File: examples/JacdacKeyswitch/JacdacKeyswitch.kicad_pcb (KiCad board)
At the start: 2 copper layers, 35 x 25 mm, 37 parts

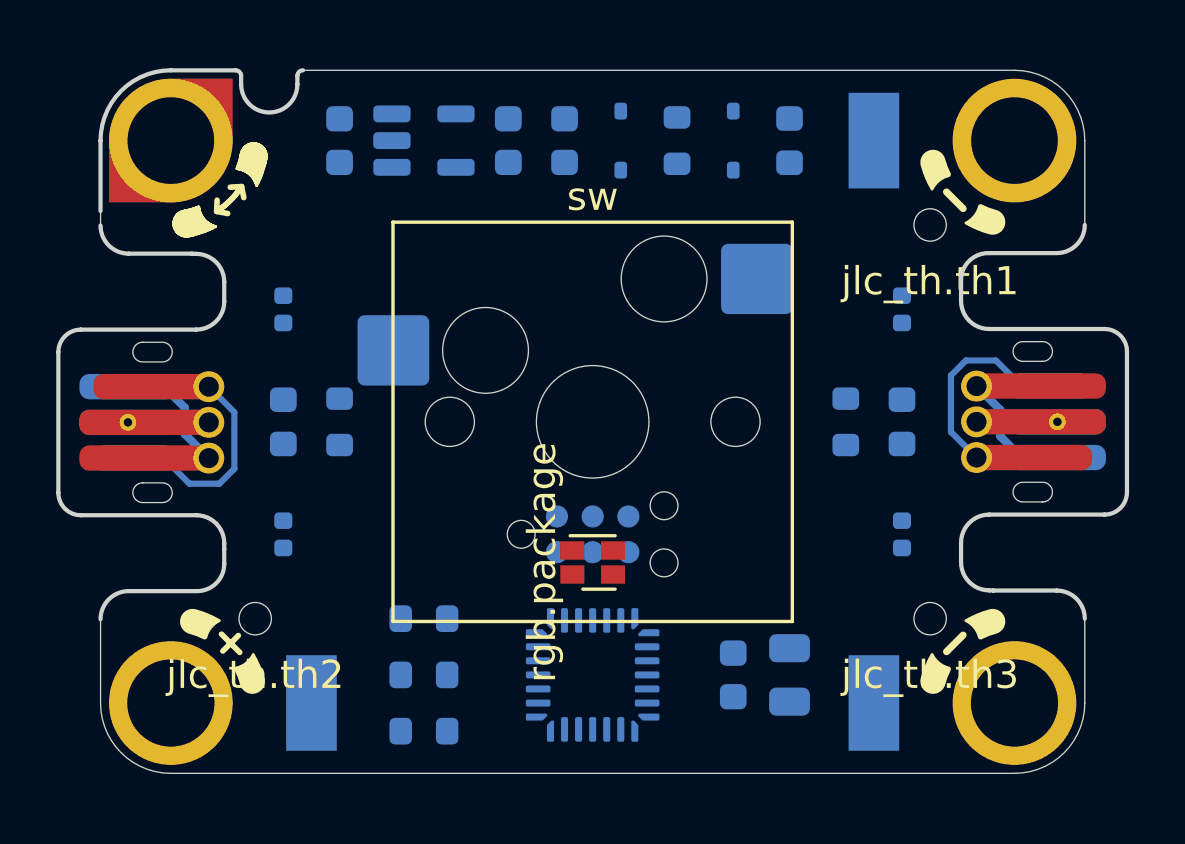
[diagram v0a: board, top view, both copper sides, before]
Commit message: layout!
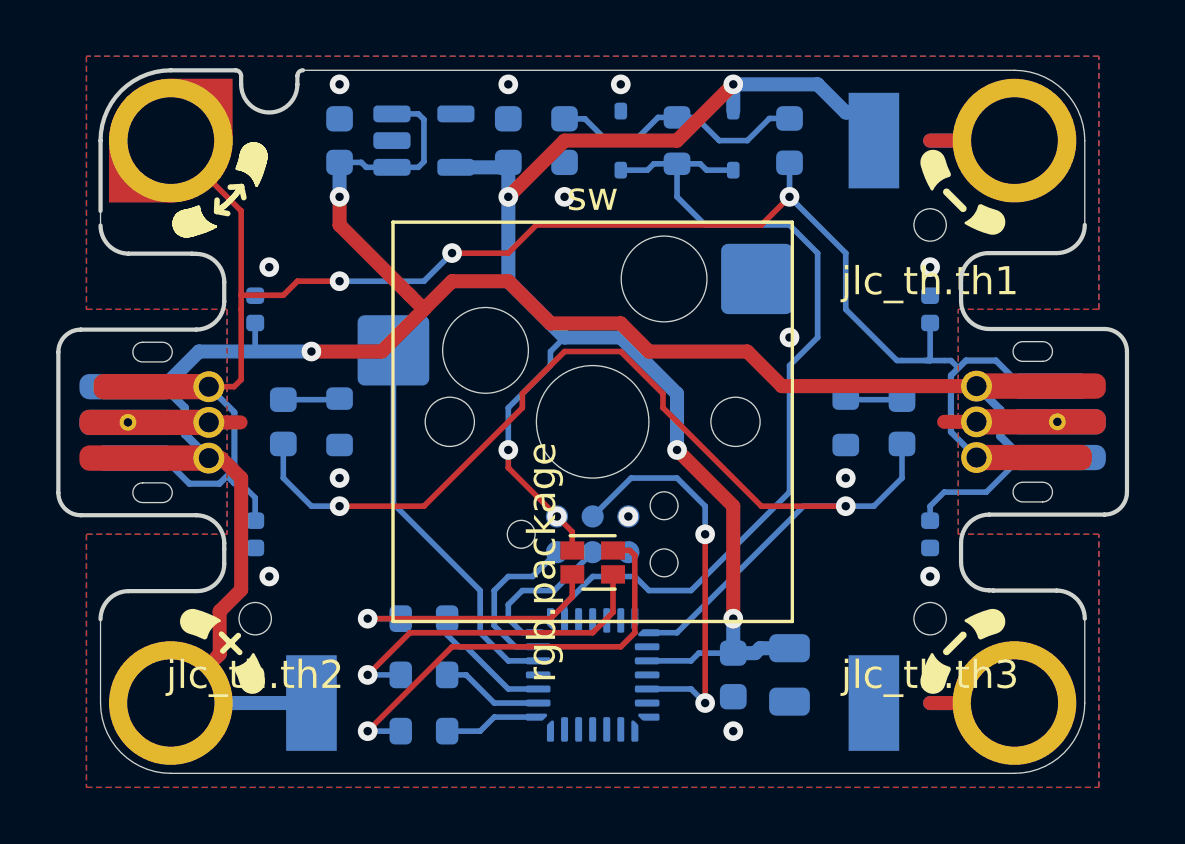
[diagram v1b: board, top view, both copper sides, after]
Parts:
- moved edge.tvs_jd_data 1.00 mm to (138.0, 104.0)
- moved edge.tvs_jd_pwr 1.00 mm to (138.0, 96.0)
- moved edge2.tvs_jd_data 1.00 mm to (162.0, 96.0)
- moved edge2.tvs_jd_pwr 1.00 mm to (162.0, 104.0)
- turned rgb.blue_res to 0 degrees
- turned rgb.green_res to 0 degrees
- turned rgb.red_res to 0 degrees
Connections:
- mcu.ic pad 13: rgb.signals.green -> (no net)
- mcu.ic pad 15: (no net) -> rgb.signals.red
- mcu.ic pad 16: rgb.signals.red -> rgb.signals.green
- mcu.ic pad 17: (no net) -> rgb.signals.blue
- mcu.ic pad 19: (no net) -> sw.out
- mcu.ic pad 2: sw.out -> (no net)
- mcu.ic pad 27: rgb.signals.blue -> (no net)
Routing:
- net jd_pwr: track 0.00 -> 69.9 mm, vias 0 -> 2
- net v3v3: track 0.00 -> 54.5 mm, vias 0 -> 6
- net jd_data.jd_data: track 0.00 -> 46.3 mm, vias 0 -> 3
- net jd_status: track 0.00 -> 39.3 mm, vias 0 -> 2
- net jd_if.signal: track 0.00 -> 30.7 mm
- net rgb.red_res.a: track 0.00 -> 15.7 mm, vias 0 -> 1
- net gnd: track 0.00 -> 14.3 mm, vias 0 -> 13
- net mcu.reset_node: track 0.00 -> 14.2 mm, vias 0 -> 2
- net sw.out: track 0.00 -> 13.8 mm
- net rgb.green_res.a: track 0.00 -> 12.2 mm, vias 0 -> 1
- net rgb.blue_res.a: track 0.00 -> 9.57 mm, vias 0 -> 1
- net jd_if.ferrite.b: track 0.00 -> 9.33 mm
- net mcu.swd_node.swdio: track 0.00 -> 5.92 mm
- net mcu.swd_node.swclk: track 0.00 -> 5.48 mm
- net rgb.signals.blue: track 0.00 -> 4.61 mm
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- added copper zone on B.Cu, net gnd
- added copper zone on F.Cu, net gnd
